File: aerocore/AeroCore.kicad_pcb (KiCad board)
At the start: 2 copper layers, 60 x 60 mm, 55 parts, among them J1 USB_C_Receptacle_USB2.0_16P, J2 Conn_ARM_JTAG_SWD_10, J3 Conn_01x02_Pin, J4 Conn_01x06_Pin, Q1 DMG3418L, U1 RP2040, U2 AP2112K-3.3, U3 MCP73831-2-OT, U4 W25Q16JVUXIQ TR, U5 BMP388, U6 LIS3MDL, U7 ICM-20649, Y2 12MHz

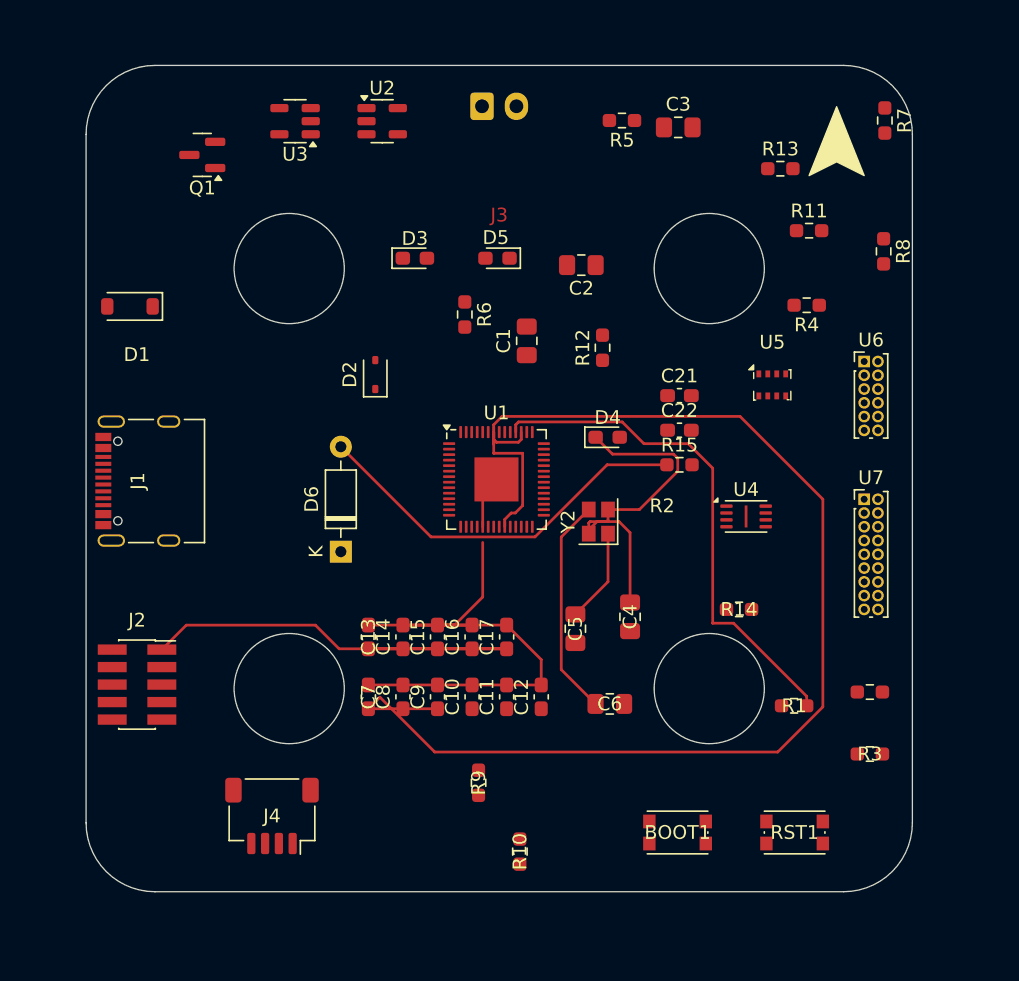
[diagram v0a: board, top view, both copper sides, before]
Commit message: add files for final board
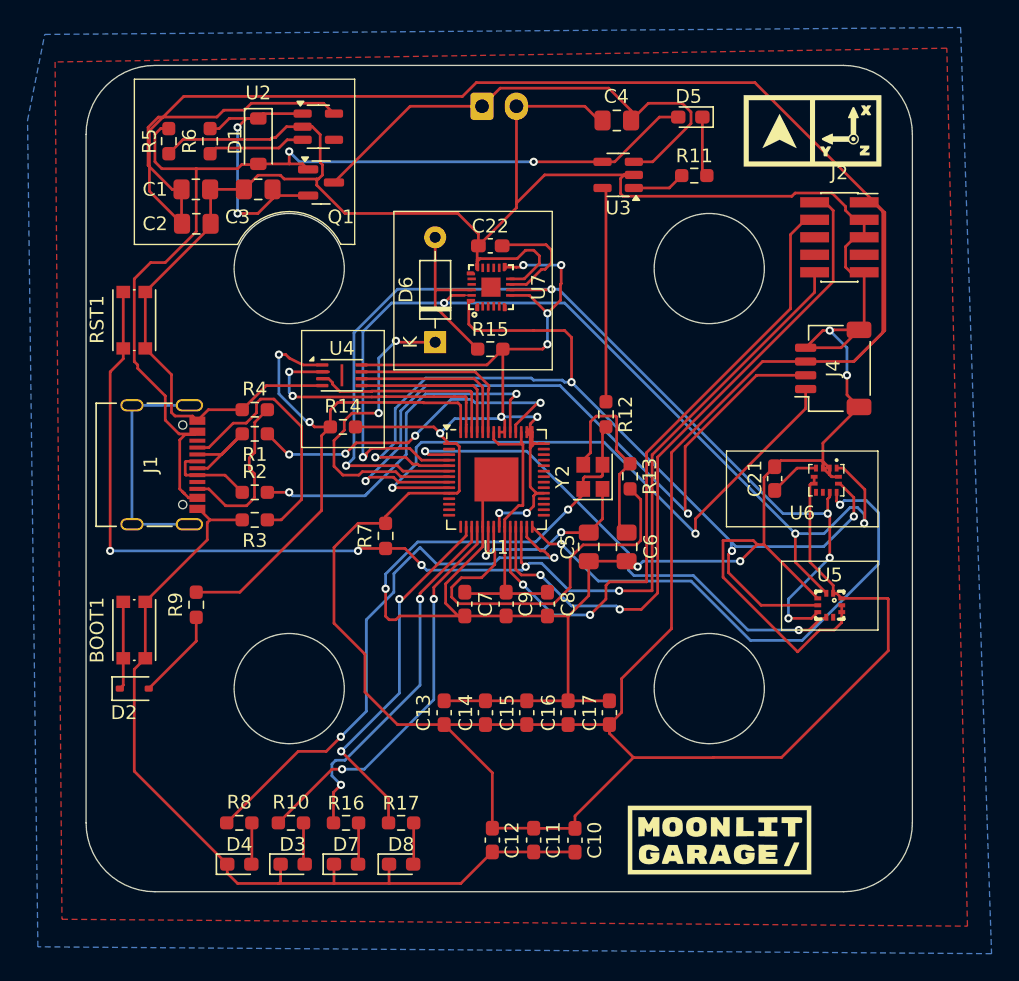
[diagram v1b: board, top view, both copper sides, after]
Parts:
- added  : LOGO, LOGO, F.Cu at (66.0, 186.2)
- added D7: RED, LED_SMD:LED_0603_1608Metric_Pad1.05x0.95mm_HandSolder, F.Cu at (38.9, 188.0)
- added D8: RED, LED_SMD:LED_0603_1608Metric_Pad1.05x0.95mm_HandSolder, F.Cu at (42.9, 188.0)
- added G***: LOGO, LOGO, F.Cu at (72.8, 134.8)
- added R16: 10k, Resistor_SMD:R_0603_1608Metric_Pad0.98x0.95mm_HandSolder, F.Cu at (38.9, 185.0)
- added R17: 10k, Resistor_SMD:R_0603_1608Metric_Pad0.98x0.95mm_HandSolder, F.Cu at (42.9, 185.0)
- U5: footprint Package_LGA:Bosch_LGA-8_2x2.5mm_P0.65mm_ClockwisePinNumbering -> easyeda2kicad:SENSORM-SMD_BMP388
- U6: footprint Connector_PinHeader_1.00mm:PinHeader_2x06_P1.00mm_Vertical -> easyeda2kicad:LGA-12_L2.0-W2.0-P0.50-BL
- U7: footprint Connector_PinHeader_1.00mm:PinHeader_2x09_P1.00mm_Vertical -> easyeda2kicad:QFN-24_L3.0-W3.0-P0.40-TL-EP1.4
- moved R8 62.5 mm to (31.1, 185.0), turned to 0 degrees
- moved RST1 60.7 mm to (23.5, 148.5), turned to 90 degrees
- moved J2 60.5 mm to (74.7, 142.5)
- moved J4 52.1 mm to (74.2, 152.0), turned to 90 degrees
- moved R3 47.8 mm to (32.2, 163.0), turned to 180 degrees
- moved R7 47.2 mm to (41.8, 164.2), turned to 90 degrees
- moved R2 47.0 mm to (32.2, 161.0)
- moved D3 44.9 mm to (35.0, 188.0)
- moved R1 43.9 mm to (32.2, 156.8)
- moved BOOT1 42.1 mm to (23.5, 171.0), turned to 90 degrees
- moved D4 40.9 mm to (31.1, 188.0)
- moved R4 40.8 mm to (32.2, 155.0), turned to 0 degrees
- moved C4 36.1 mm to (58.5, 134.0), turned to 180 degrees
- moved R5 32.9 mm to (26.0, 135.5), turned to -90 degrees
- moved R14 31.7 mm to (38.6, 156.2)
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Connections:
- R10 pad 1: /D13 -> /D15
- R8 pad 1: /D14 -> /D16
- U1 pad 28: /D17 -> /CS_3
- U1 pad 3: /D1 -> /CS_2
- U1 pad 4: /D2 -> /SCK0
- U1 pad 5: /D3 -> /MOSI0
- U1 pad 6: /D4 -> /MISO0
- U1 pad 7: /D5 -> /CS_1
- U1 pad 8: /D6 -> /SDA
- U1 pad 9: /D7 -> /SCL
- U5 pad 2: /SCK -> /SCK0
- U5 pad 4: /MOSI -> /MOSI0
- U5 pad 5: /MISO -> /MISO0
- U6 pad 1: /SCK -> /SCK0
- U6 pad 11: /MOSI -> /MOSI0
- U6 pad 9: /MISO -> /MISO0
- U7 pad 9: /MISO -> /MISO0
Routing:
- net /+3v3: track 36.5 -> 325.3 mm, vias 0 -> 9
- net GND: track 70.6 -> 349.7 mm, vias 0 -> 6
- net /~{RESET}: track 0.00 -> 91.4 mm, vias 0 -> 5
- net /VBUS: track 0.00 -> 77.0 mm, vias 0 -> 2
- net /1.2V: track 97.4 -> 21.2 mm
- net /MISO0: track 0.00 -> 76.1 mm, vias 0 -> 5
- net /MOSI0: track 0.00 -> 75.7 mm, vias 0 -> 4
- net /SCK0: track 0.00 -> 74.6 mm, vias 0 -> 4
- net /SDA: track 0.00 -> 53.8 mm, vias 0 -> 2
- net /SWDIO: track 0.00 -> 50.4 mm, vias 0 -> 2
- net /SWCLK: track 0.00 -> 47.8 mm, vias 0 -> 2
- net /SCL: track 0.00 -> 44.8 mm, vias 0 -> 2
- net /D16: track 0.00 -> 40.8 mm, vias 0 -> 2
- net /QSPI_CS: track 0.00 -> 39.3 mm, vias 0 -> 2
- net /CS_3: track 0.00 -> 38.9 mm, vias 0 -> 2
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- added copper zone on B.Cu, net GND
- added copper zone on F.Cu, net GND
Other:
- board text added: "Aeronode"
- board text added: "v0.0.1"
- board text removed: "AeroNode"
